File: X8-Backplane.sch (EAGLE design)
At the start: 3 parts

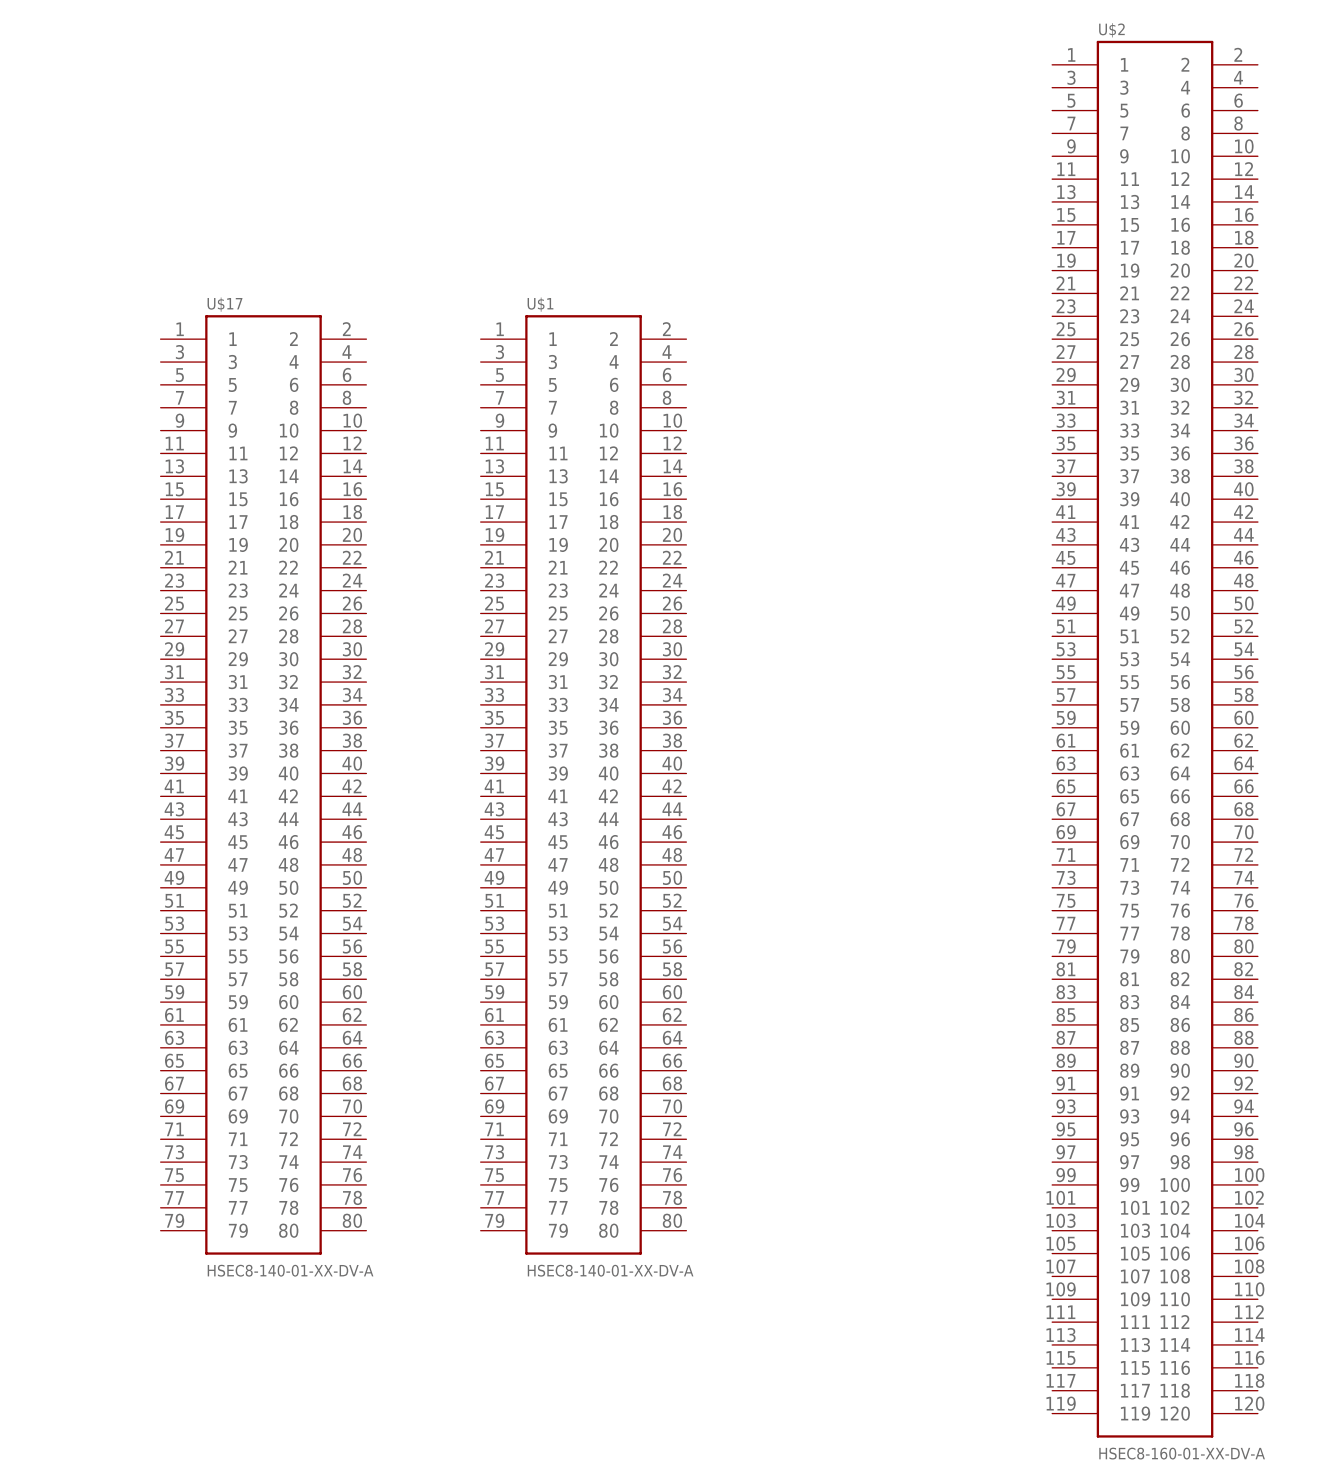
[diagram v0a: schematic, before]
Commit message: Fleshing out the idea for the backplane
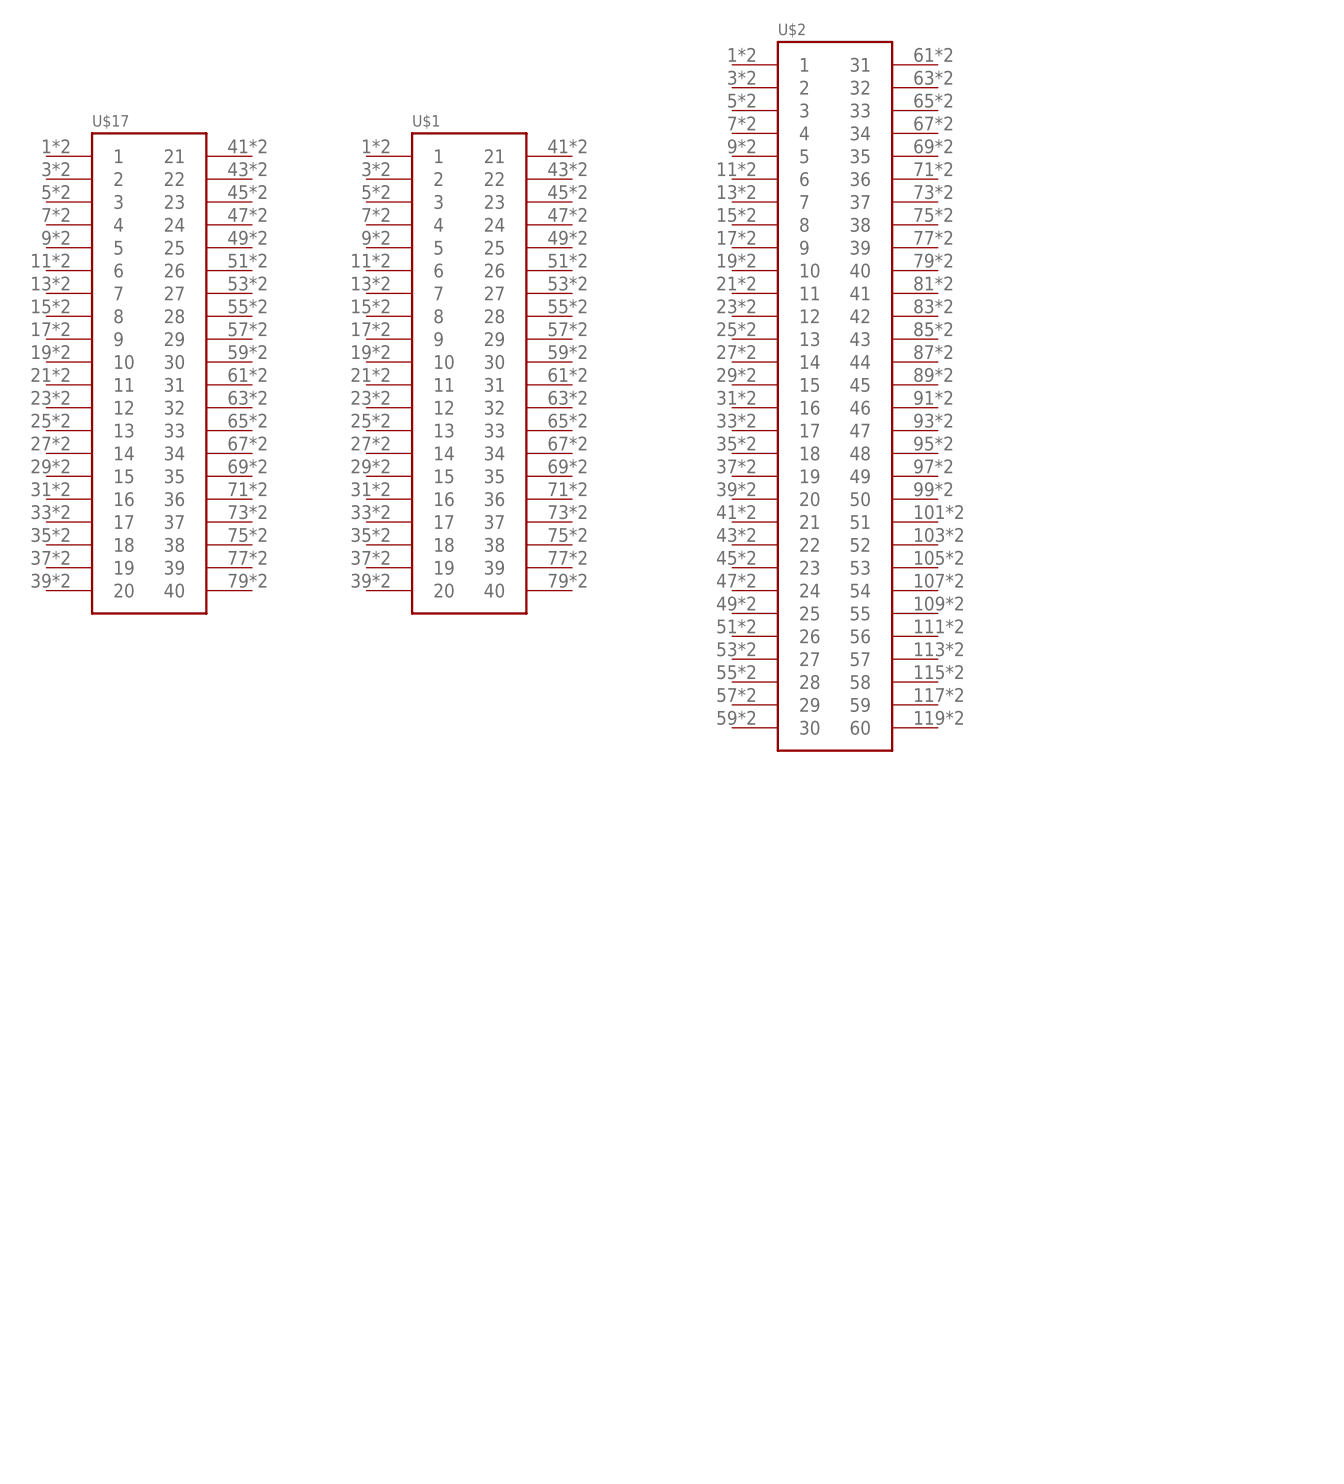
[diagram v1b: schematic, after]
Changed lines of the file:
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@@
 <part name="FRAME1" library="frames" deviceset="A4-SMALL-DOCFIELD" device=""/>
 <part name="U$1" library="HSEC8-1xx-01-XX-DV-A" deviceset="HSEC8-140-01-XX-DV-A" device=""/>
+<part name="U$17" library="HSEC8-1xx-01-XX-DV-A" deviceset="HSEC8-140-01-XX-DV-A" device=""/>
 <part name="U$2" library="HSEC8-1xx-01-XX-DV-A" deviceset="HSEC8-160-01-XX-DV-A" device=""/>
-<part name="U$17" library="HSEC8-1xx-01-XX-DV-A" deviceset="HSEC8-140-01-XX-DV-A" device=""/>
 </parts>
 <sheets>
@@
 <instance part="FRAME1" gate="/1" x="0" y="0"/>
 <instance part="U$1" gate="G$1" x="50.8" y="190.5"/>
-<instance part="U$2" gate="G$1" x="114.3" y="220.98"/>
 <instance part="U$17" gate="G$1" x="15.24" y="190.5"/>
+<instance part="U$2" gate="G$1" x="91.44" y="185.42"/>
 </instances>
 <busses>
